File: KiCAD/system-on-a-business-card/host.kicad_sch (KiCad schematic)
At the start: 27 parts, among them Q1 2N7002K, Q2 2N7002K, SW2 SW_Push, U2 ESP32-C3, U3 ZD25WQ32C, Y1 40MHz

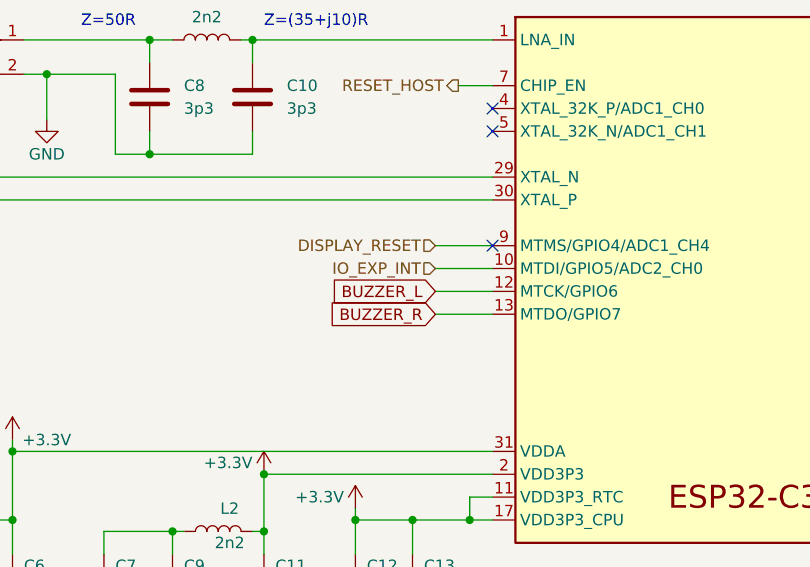
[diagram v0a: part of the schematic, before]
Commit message: #10: started with routing
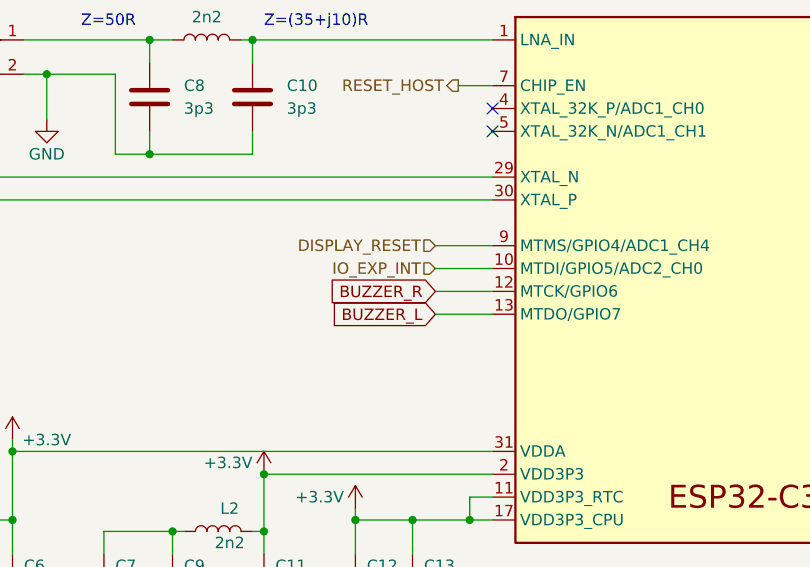
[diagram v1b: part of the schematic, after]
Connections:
- net BUZZER_L: now also U2.13 (MTDO/GPIO7); no longer U2.12 (MTCK/GPIO6)
- net BUZZER_R: now also U2.12 (MTCK/GPIO6); no longer U2.13 (MTDO/GPIO7)
- no-connect marks 5 -> 4
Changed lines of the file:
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@@
   (no_connect (at 182.88 77.47))
   (no_connect (at 127 39.37))
-  (no_connect (at 127 54.61))
   (no_connect (at 182.88 74.93))
   (no_connect (at 127 41.91))
@@
     )
   )
-  (global_label "BUZZER_R" (shape input) (at 120.65 62.23 180) (fields_autoplaced)
+  (global_label "BUZZER_R" (shape input) (at 120.65 59.69 180) (fields_autoplaced)
     (effects (font (size 1.27 1.27)) (justify right))
-    (property "Intersheetrefs" "${INTERSHEET_REFS}" (at 107.9887 62.23 0)
+    (property "Intersheetrefs" "${INTERSHEET_REFS}" (at 107.9887 59.69 0)
       (effects (font (size 1.27 1.27)) (justify right) hide)
     )
@@
     )
   )
-  (global_label "BUZZER_L" (shape input) (at 120.65 59.69 180) (fields_autoplaced)
+  (global_label "BUZZER_L" (shape input) (at 120.65 62.23 180) (fields_autoplaced)
     (effects (font (size 1.27 1.27)) (justify right))
-    (property "Intersheetrefs" "${INTERSHEET_REFS}" (at 108.2306 59.69 0)
+    (property "Intersheetrefs" "${INTERSHEET_REFS}" (at 108.2306 62.23 0)
       (effects (font (size 1.27 1.27)) (justify right) hide)
     )
